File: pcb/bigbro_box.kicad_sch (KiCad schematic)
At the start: 47 parts, among them J1 Current Sense, J2 Display, J3 Mains, J4 Debug, J5 RFID, J6 Relay, J7 Ext, K1 G5LE-1, Q1 MMBT3904, Q2 MMBT3904, Q3 BSS138, Q4 MMBT3906, SW1 Card switch, SW2 SW_SPST, SW3 SW_SPST, U1 ESP32-WROOM-32, U2 AP1117-33, U3 4011, U4 4011, U5 RDM6300

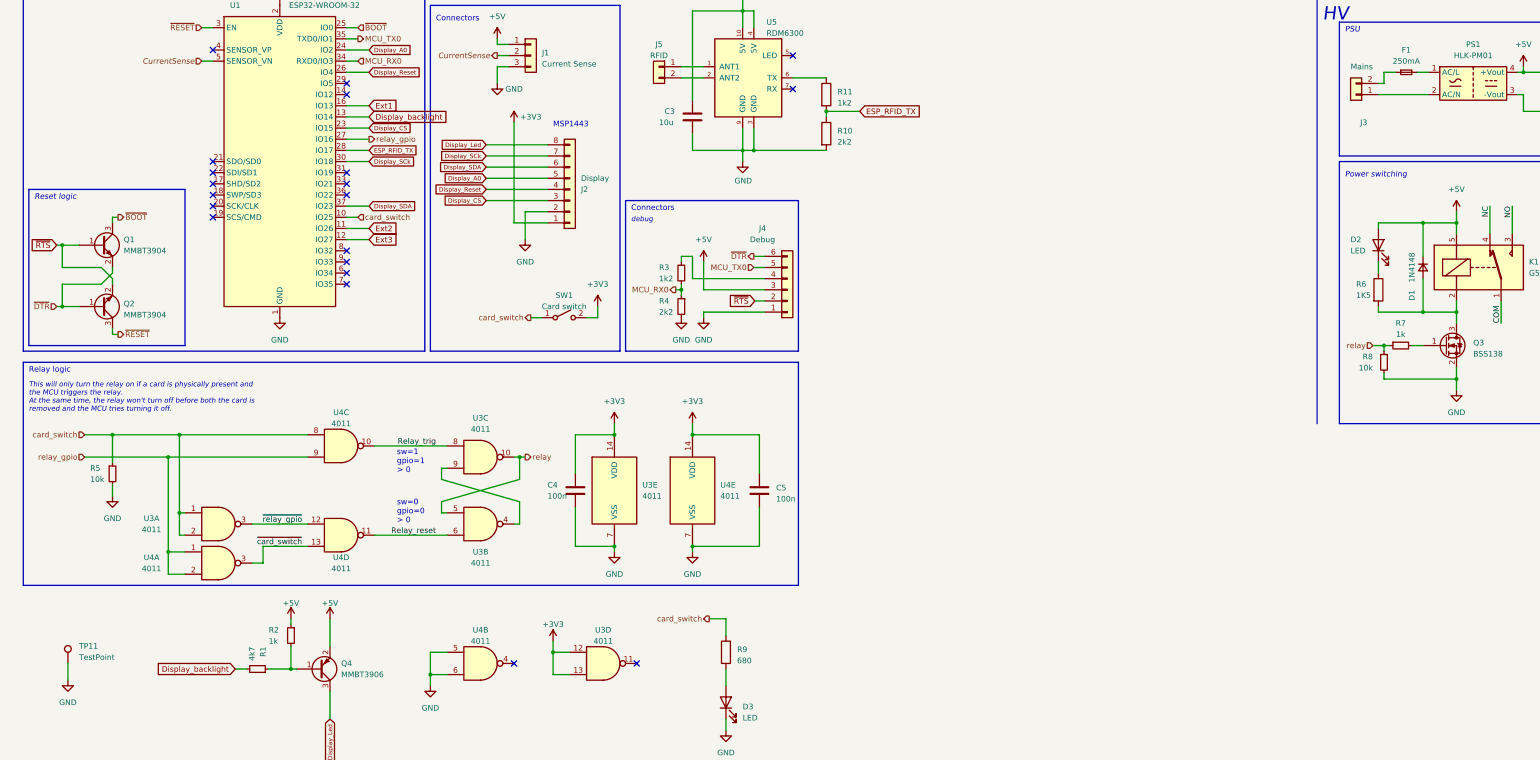
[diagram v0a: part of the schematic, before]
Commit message: Add schematic.
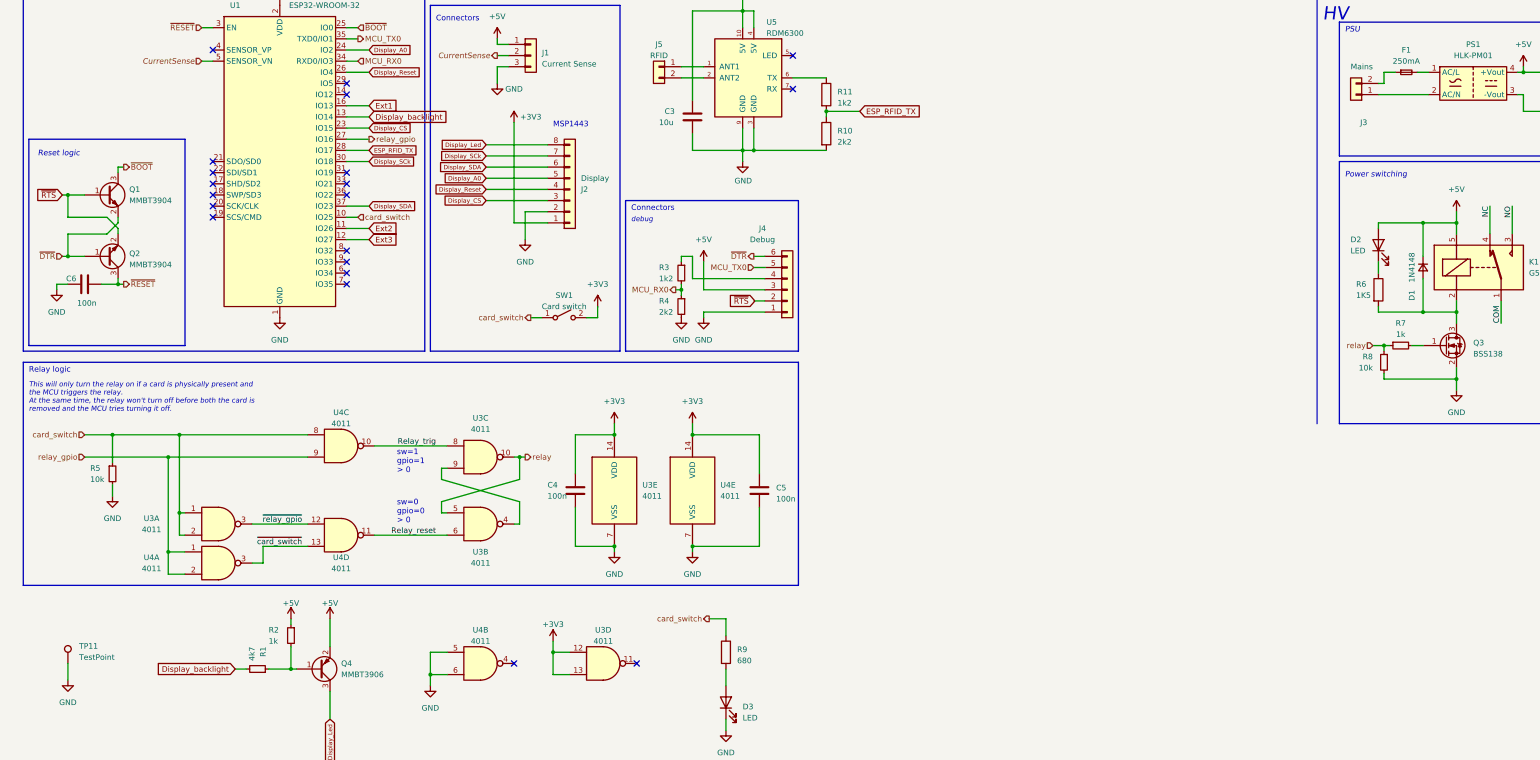
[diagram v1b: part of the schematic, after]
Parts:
- added C6: 100n, Capacitor_SMD:C_0603_1608Metric, symbol Device:C
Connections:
- net GND: now also C6.2
- net ~{RESET}: now also C6.1
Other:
- moved on the sheet: Q1, Q2

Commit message: Change C3 to 0608.
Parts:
- C3: footprint Capacitor_SMD:C_0805_2012Metric -> Capacitor_SMD:C_0603_1608Metric
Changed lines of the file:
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@@
 			)
 		)
-		(property "Footprint" "Capacitor_SMD:C_0805_2012Metric"
+		(property "Footprint" "Capacitor_SMD:C_0603_1608Metric"
 			(at 168.6052 53.34 0)
 			(effects
